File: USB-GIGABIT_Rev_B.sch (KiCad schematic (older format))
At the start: 49 parts, among them P1 USB_C_Plug, U2 n.a.(93LC46), U3 RTL8153VCCG, U4 SY8089AAAC(SOT23-5), X1 SMD РЕЗ. 3225 25 Mhz 20 pf 20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

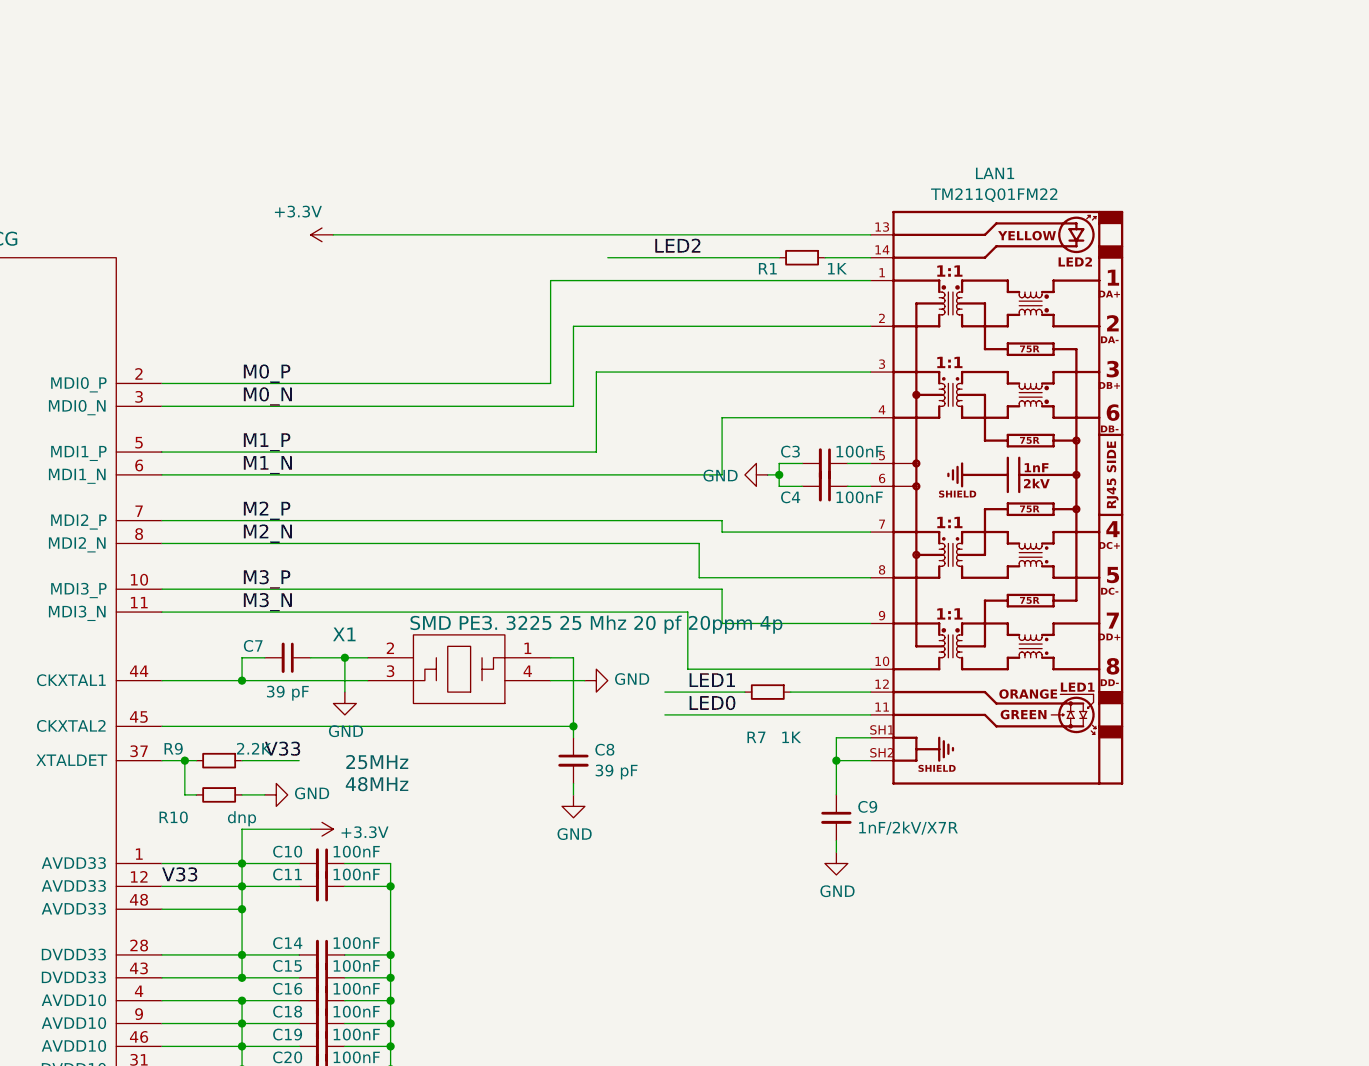
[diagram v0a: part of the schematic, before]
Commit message: Updated to Newest change.
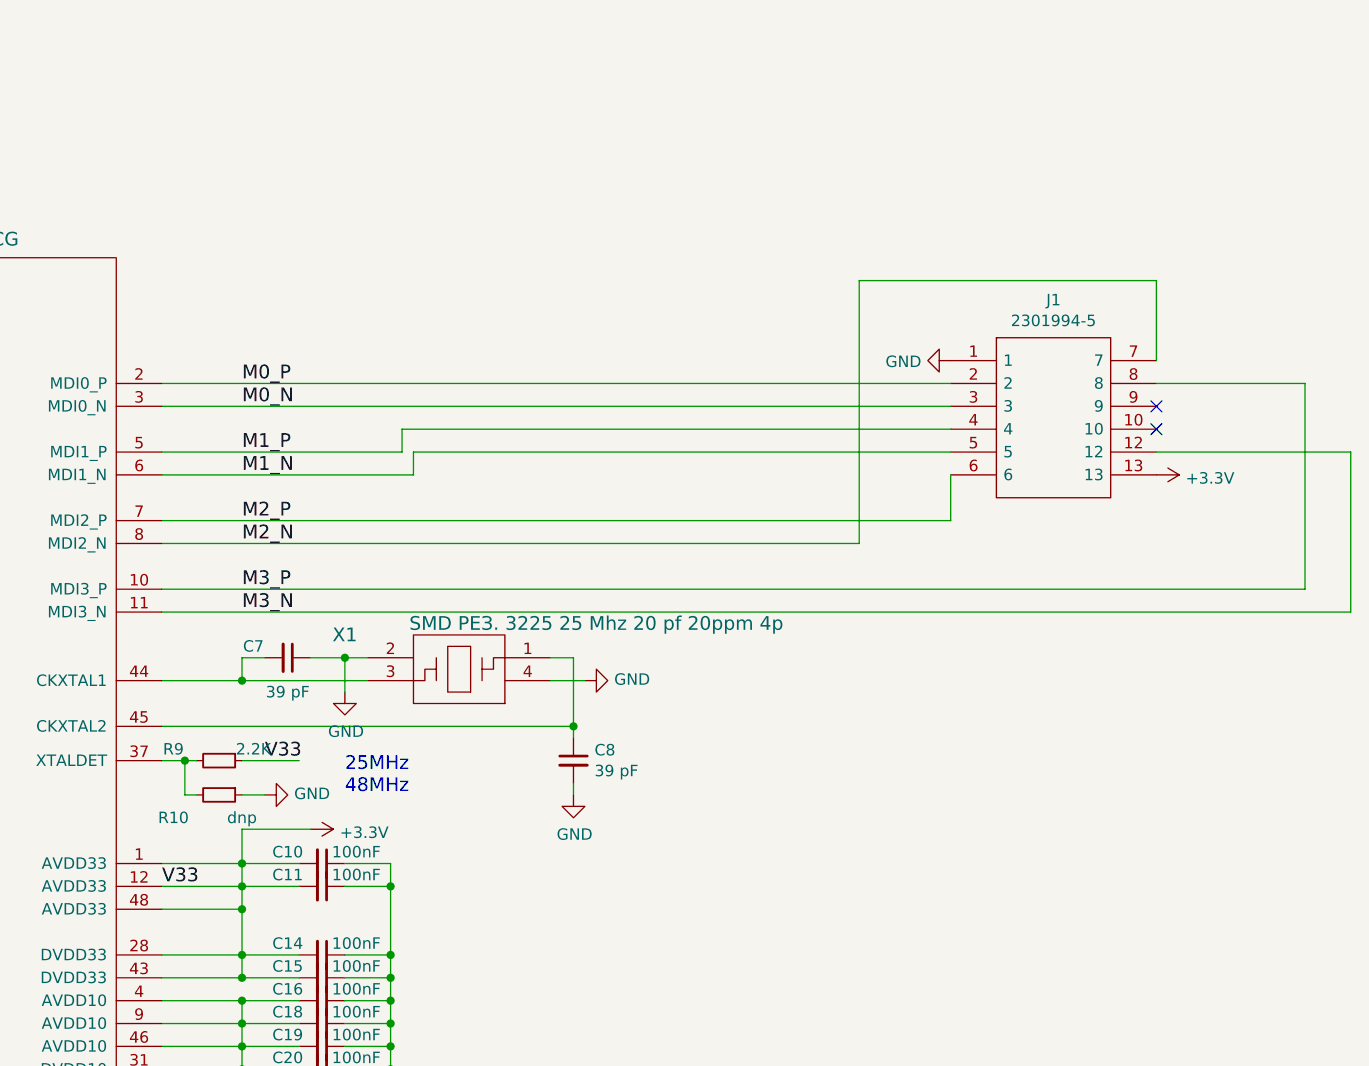
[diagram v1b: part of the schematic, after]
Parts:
- removed C3, C4: 100nF, OLIMEX_RLC-FP:C_0805_5MIL_DWS, symbol USB-GIGABIT_Rev_B-rescue:C_Small-USB-GIGABIT_Rev_C
- removed C9: 1nF/2kV/X7R, OLIMEX_RLC-FP:C_1206_5MIL_DWS_ISO, symbol USB-GIGABIT_Rev_B-rescue:C_Small-USB-GIGABIT_Rev_C
- removed LAN1: TM211Q01FM22, OLIMEX_Connectors-FP:TM211Q01FM22, symbol USB-GIGABIT_Rev_B-rescue:TM211Q01FM22-USB-GIGABIT_Rev_C
- removed R1, R7: 1K, OLIMEX_RLC-FP:R_0603_5MIL_DWS, symbol USB-GIGABIT_Rev_B-rescue:R_Small-USB-GIGABIT_Rev_C
- added J1: 2301994-5, 23019945, symbol SamacSys_Parts:2301994-5
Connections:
- net +3V3: now also J1.13
- net GND: now also J1.1
- net M0_N: now also J1.3
- net M0_P: now also J1.2
- net M1_N: now also J1.5
- net M1_P: now also J1.4
- net M2_N: now also J1.7
- net M2_P: now also J1.6
- net M3_N: now also J1.12
- net M3_P: now also J1.8
- no-connect marks 4 -> 6
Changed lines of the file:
@@
 	1    0    0    -1
 $EndComp
-Wire Wire Line
-	8750 3400 9100 3400
-Wire Wire Line
-	8500 1500 9250 1500
-Text Label 8700 1500 0    60   ~ 0
-LED2
 Text Label 4450 2800 0    60   ~ 0
 LED2
-$Comp
-L USB-GIGABIT_Rev_B-rescue:+3.3V-USB-GIGABIT_Rev_C #PWR0103
-U 1 1 5D7650F9
-P 7300 1400
-F 0 "#PWR0103" H 7300 1250 50  0001 C CNN
-F 1 "+3.3V" V 7400 1450 50  0000 L CNN
-F 2 "" H 7300 1400 60  0000 C CNN
-F 3 "" H 7300 1400 60  0000 C CNN
-	1    7300 1400
-	0    -1   -1   0
-$EndComp
 Wire Wire Line
 	1400 5250 2000 5250
@@
 Wire Wire Line
 	800  3800 950  3800
-Wire Wire Line
-	9250 2450 9250 2500
-Wire Wire Line
-	9500 3700 9500 3850
 Wire Wire Line
 	4050 5550 4050 4850
@@
 U3SRX_P
 NoConn ~ 4400 2500
-Wire Wire Line
-	9650 3500 8750 3500
-Text Label 8850 3400 0    60   ~ 0
-LED1
 Text Label 4500 3000 0    60   ~ 0
 LED1
@@
 Wire Wire Line
 	4700 2700 4400 2700
-Text Label 8850 3500 0    60   ~ 0
-LED0
 $Comp
 L USB-GIGABIT_Rev_B-rescue:GND-USB-GIGABIT_Rev_C #PWR015
@@
 	1    0    0    -1
 $EndComp
-Wire Wire Line
-	9300 3400 9650 3400
-$Comp
-L USB-GIGABIT_Rev_B-rescue:R_Small-USB-GIGABIT_Rev_C R7
-U 1 1 5942907E
-P 9200 3400
-F 0 "R7" V 9400 3350 50  0000 C CNN
-F 1 "1K" V 9400 3500 50  0000 C CNN
-F 2 "OLIMEX_RLC-FP:R_0603_5MIL_DWS" H 9200 3400 60  0001 C CNN
-F 3 "" H 9200 3400 60  0000 C CNN
-	1    9200 3400
-	0    1    1    0
-$EndComp
-$Comp
-L USB-GIGABIT_Rev_B-rescue:R_Small-USB-GIGABIT_Rev_C R1
-U 1 1 59428F99
-P 9350 1500
-F 0 "R1" V 9400 1350 50  0000 C CNN
-F 1 "1K" V 9400 1650 50  0000 C CNN
-F 2 "OLIMEX_RLC-FP:R_0603_5MIL_DWS" H 9350 1500 60  0001 C CNN
-F 3 "" H 9350 1500 60  0000 C CNN
-	1    9350 1500
-	0    1    1    0
-$EndComp
-Wire Wire Line
-	9650 1500 9450 1500
-Wire Wire Line
-	7300 1400 9650 1400
-$Comp
-L USB-GIGABIT_Rev_B-rescue:GND-USB-GIGABIT_Rev_C #PWR02
-U 1 1 59428D23
-P 9200 2450
-F 0 "#PWR02" H 9200 2200 50  0001 C CNN
-F 1 "GND" V 9205 2322 50  0000 R CNN
-F 2 "" H 9200 2450 60  0000 C CNN
-F 3 "" H 9200 2450 60  0000 C CNN
-	1    9200 2450
-	0    1    1    0
-$EndComp
-Wire Wire Line
-	9250 2450 9200 2450
-Wire Wire Line
-	9250 2400 9350 2400
-Connection ~ 9250 2450
-Wire Wire Line
-	9250 2400 9250 2450
-Wire Wire Line
-	9250 2500 9350 2500
-Wire Wire Line
-	9650 2500 9550 2500
-Wire Wire Line
-	9550 2400 9650 2400
-$Comp
-L USB-GIGABIT_Rev_B-rescue:C_Small-USB-GIGABIT_Rev_C C4
-U 1 1 59428C3F
-P 9450 2500
-F 0 "C4" V 9500 2350 50  0000 C CNN
-F 1 "100nF" V 9500 2650 50  0000 C CNN
-F 2 "OLIMEX_RLC-FP:C_0805_5MIL_DWS" H 9450 2500 60  0001 C CNN
-F 3 "" H 9450 2500 60  0000 C CNN
-	1    9450 2500
-	0    1    1    0
-$EndComp
-$Comp
-L USB-GIGABIT_Rev_B-rescue:C_Small-USB-GIGABIT_Rev_C C3
-U 1 1 59428C02
-P 9450 2400
-F 0 "C3" V 9400 2250 50  0000 C CNN
-F 1 "100nF" V 9400 2550 50  0000 C CNN
-F 2 "OLIMEX_RLC-FP:C_0805_5MIL_DWS" H 9450 2400 60  0001 C CNN
-F 3 "" H 9450 2400 60  0000 C CNN
-	1    9450 2400
-	0    1    1    0
-$EndComp
-$Comp
-L USB-GIGABIT_Rev_B-rescue:GND-USB-GIGABIT_Rev_C #PWR01
-U 1 1 59428BB3
-P 9500 4100
-F 0 "#PWR01" H 9500 3850 50  0001 C CNN
-F 1 "GND" H 9505 3927 50  0000 C CNN
-F 2 "" H 9500 4100 60  0000 C CNN
-F 3 "" H 9500 4100 60  0000 C CNN
-	1    9500 4100
-	1    0    0    -1
-$EndComp
-Wire Wire Line
-	9500 4050 9500 4100
-$Comp
-L USB-GIGABIT_Rev_B-rescue:C_Small-USB-GIGABIT_Rev_C C9
-U 1 1 59428B53
-P 9500 3950
-F 0 "C9" H 9592 3996 50  0000 L CNN
-F 1 "1nF/2kV/X7R" H 9592 3905 50  0000 L CNN
-F 2 "OLIMEX_RLC-FP:C_1206_5MIL_DWS_ISO" H 9500 3950 60  0001 C CNN
-F 3 "" H 9500 3950 60  0000 C CNN
-	1    9500 3950
-	1    0    0    -1
-$EndComp
-Wire Wire Line
-	9650 3700 9500 3700
-Connection ~ 9500 3700
-Wire Wire Line
-	9500 3600 9500 3700
-Wire Wire Line
-	9650 3600 9500 3600
-Wire Wire Line
-	8850 3050 6550 3050
-Wire Wire Line
-	8850 3300 8850 3050
-Wire Wire Line
-	9650 3300 8850 3300
-Wire Wire Line
-	9000 3100 9650 3100
-Wire Wire Line
-	9000 2950 9000 3100
-Wire Wire Line
-	6550 2950 9000 2950
-Wire Wire Line
-	8900 2750 6550 2750
-Wire Wire Line
-	8900 2900 8900 2750
-Wire Wire Line
-	9650 2900 8900 2900
-Wire Wire Line
-	9000 2700 9650 2700
-Wire Wire Line
-	9000 2650 9000 2700
-Wire Wire Line
-	6550 2650 9000 2650
-Wire Wire Line
-	9000 2450 6550 2450
-Wire Wire Line
-	9000 2200 9000 2450
-Wire Wire Line
-	9650 2200 9000 2200
-Wire Wire Line
-	8450 2000 9650 2000
-Wire Wire Line
-	8450 2350 8450 2000
-Wire Wire Line
-	6550 2350 8450 2350
-Wire Wire Line
-	8350 2150 6550 2150
-Wire Wire Line
-	8350 1800 8350 2150
-Wire Wire Line
-	9650 1800 8350 1800
-Wire Wire Line
-	8250 1600 9650 1600
-Wire Wire Line
-	8250 2050 8250 1600
-Wire Wire Line
-	6550 2050 8250 2050
-$Comp
-L USB-GIGABIT_Rev_B-rescue:TM211Q01FM22-USB-GIGABIT_Rev_C LAN1
-U 1 1 594283EE
-P 10250 2500
-F 0 "LAN1" H 10306 3867 50  0000 C CNN
-F 1 "TM211Q01FM22" H 10306 3776 50  0000 C CNN
-F 2 "OLIMEX_Connectors-FP:TM211Q01FM22" H 10280 2650 20  0001 C CNN
-F 3 "" H 10250 2500 60  0000 C CNN
-	1    10250 2500
-	-1   0    0    -1
-$EndComp
 $Comp
 L USB-GIGABIT_Rev_B-rescue:RTL8153VCCG-USB-GIGABIT_Rev_C U3
@@
 Text Notes 10600 7650 0    60   ~ 0
 B\n
+$Comp
+L power:+3.3V #PWR0104
+U 1 1 61A02D1D
+P 10900 2450
+F 0 "#PWR0104" H 10900 2300 50  0001 C CNN
+F 1 "+3.3V" V 10915 2578 50  0000 L CNN
+F 2 "" H 10900 2450 50  0001 C CNN
+F 3 "" H 10900 2450 50  0001 C CNN
+	1    10900 2450
+	0    1    1    0
+$EndComp
+$Comp
+L SamacSys_Parts:2301994-5 J1
+U 1 1 619C224D
+P 10000 1950
+F 0 "J1" H 10450 2215 50  0000 C CNN
+F 1 "2301994-5" H 10450 2124 50  0000 C CNN
+F 2 "23019945" H 10750 2050 50  0001 L CNN
+F 3 "https://www.te.com/commerce/DocumentDelivery/DDEController?Action=srchrtrv&DocNm=2301994-5&DocType=Customer+Drawing&DocLang=English&DocFormat=pdf&PartCntxt=2301994-5" H 10750 1950 50  0001 L CNN
+F 4 "TE CONNECTIVITY - 2301994-5 - RJ45 CONNECTOR, JACK, 8P8C, 1PORT, TH" H 10750 1850 50  0001 L CNN "Description"
+F 5 "17.3" H 10750 1750 50  0001 L CNN "Height"
+F 6 "TE Connectivity" H 10750 1650 50  0001 L CNN "Manufacturer_Name"
+F 7 "2301994-5" H 10750 1550 50  0001 L CNN "Manufacturer_Part_Number"
+F 8 "571-2301994-5" H 10750 1450 50  0001 L CNN "Mouser Part Number"
+F 9 "https://www.mouser.co.uk/ProductDetail/TE-Connectivity/2301994-5?qs=u4fy%2FsgLU9MhDQYKS1KhdQ%3D%3D" H 10750 1350 50  0001 L CNN "Mouser Price/Stock"
+F 10 "2301994-5" H 10750 1250 50  0001 L CNN "Arrow Part Number"
+F 11 "https://www.arrow.com/en/products/2301994-5/te-connectivity?region=nac" H 10750 1150 50  0001 L CNN "Arrow Price/Stock"
+	1    10000 1950
+	1    0    0    -1
+$EndComp
+$Comp
+L power:GND #PWR0103
+U 1 1 61A8E398
+P 10000 1950
+F 0 "#PWR0103" H 10000 1700 50  0001 C CNN
+F 1 "GND" V 10005 1822 50  0000 R CNN
+F 2 "" H 10000 1950 50  0001 C CNN
+F 3 "" H 10000 1950 50  0001 C CNN
+	1    10000 1950
+	0    1    1    0
+$EndComp
+NoConn ~ 10900 2150
+NoConn ~ 10900 2250
+Wire Wire Line
+	6550 2050 10000 2050
+Wire Wire Line
+	6550 2150 10000 2150
+Wire Wire Line
+	7600 2350 7600 2250
+Wire Wire Line
+	7600 2250 10000 2250
+Wire Wire Line
+	6550 2350 7600 2350
+Wire Wire Line
+	7650 2450 7650 2350
+Wire Wire Line
+	7650 2350 10000 2350
+Wire Wire Line
+	6550 2450 7650 2450
+Wire Wire Line
+	10000 2650 10000 2450
+Wire Wire Line
+	6550 2650 10000 2650
+Wire Wire Line
+	9600 2750 9600 1600
+Wire Wire Line
+	9600 1600 10900 1600
+Wire Wire Line
+	10900 1600 10900 1950
+Wire Wire Line
+	6550 2750 9600 2750
+Wire Wire Line
+	11550 2950 11550 2050
+Wire Wire Line
+	11550 2050 10900 2050
+Wire Wire Line
+	6550 2950 11550 2950
+Wire Wire Line
+	11750 3050 11750 2350
+Wire Wire Line
+	11750 2350 10900 2350
+Wire Wire Line
+	6550 3050 11750 3050
 $EndSCHEMATC
